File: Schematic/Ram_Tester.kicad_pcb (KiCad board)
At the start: 2 copper layers, 37.6 x 58.5 mm, 19 parts, among them J1 Conn_01x02_Pin, J2 ICSP, SW1 SW_DIP_x03, U1 ATmega328-P, U2 RAM, Y1 Crystal

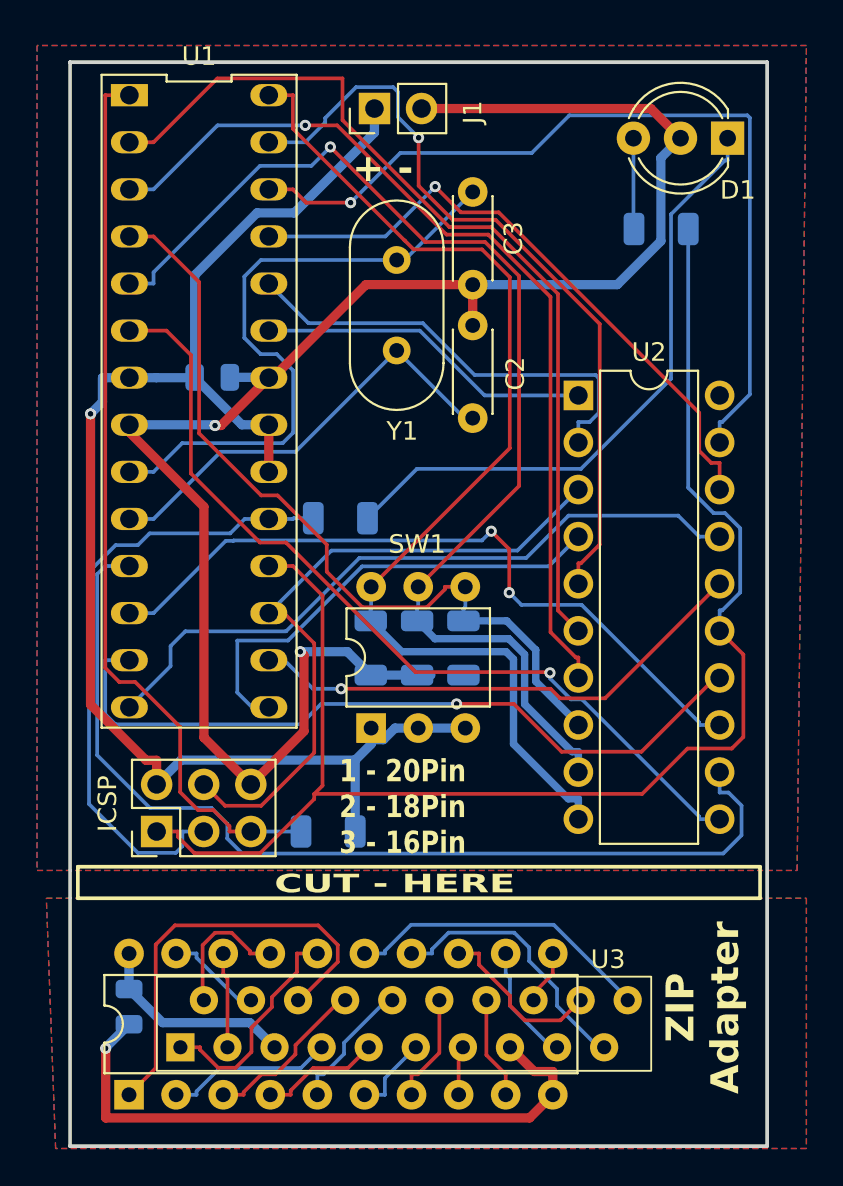
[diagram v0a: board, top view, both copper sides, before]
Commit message: v1.0 of PCB
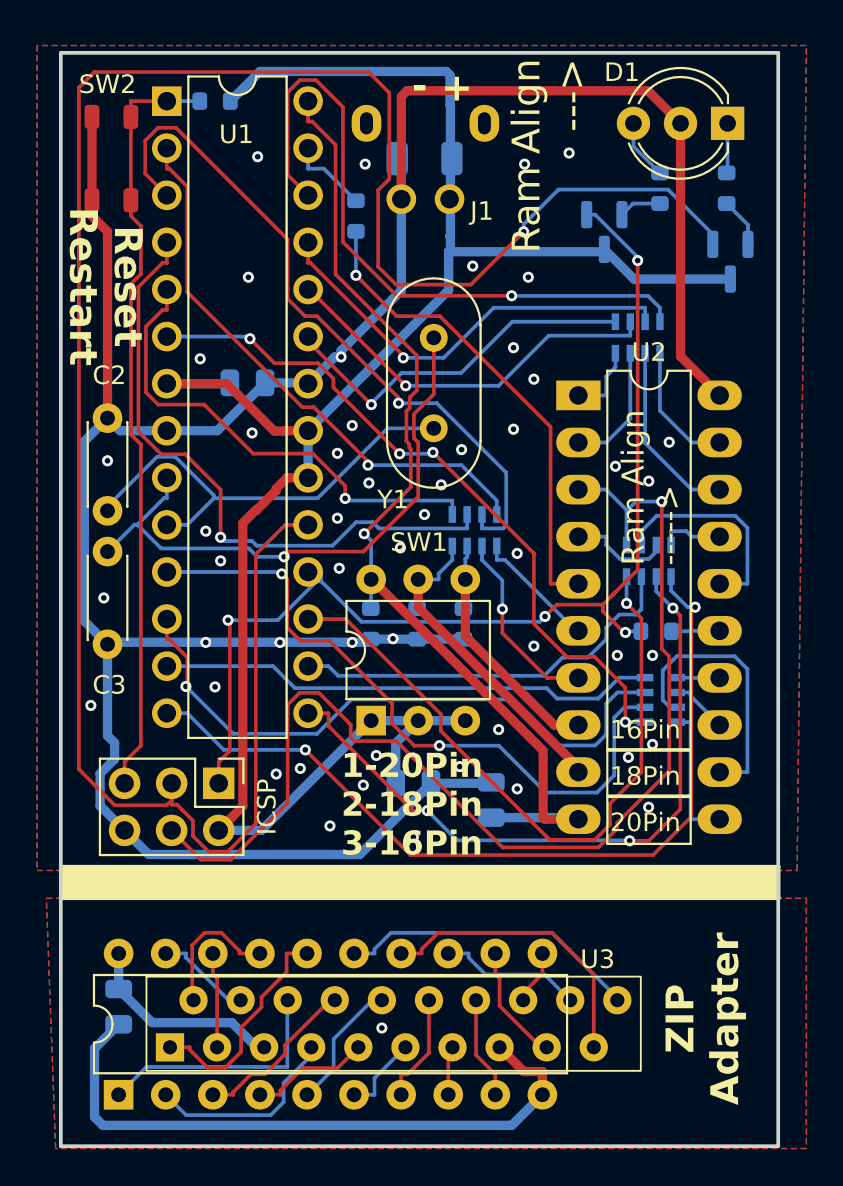
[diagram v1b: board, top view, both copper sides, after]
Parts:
- added C5: 10uF, Capacitor_SMD:C_1206_3216Metric, B.Cu at (124.9, 70.1)
- added C6: 100nF, Capacitor_SMD:C_0805_2012Metric, B.Cu at (128.5, 104.7)
- added C7: 100nF, Capacitor_SMD:C_0805_2012Metric, B.Cu at (124.3, 103.8)
- added Q1: IRLML6402, Package_TO_SOT_SMD:SOT-23, B.Cu at (134.6, 74.1)
- added Q2: IRLML6402, Package_TO_SOT_SMD:SOT-23, B.Cu at (141.4, 75.7)
- added R7: 47, Resistor_SMD:R_0603_1608Metric, B.Cu at (137.4, 95.6)
- added R8: 47, Resistor_SMD:R_0603_1608Metric, B.Cu at (121.2, 73.2)
- added RN1: 47, Resistor_SMD:R_Array_Concave_4x0603, B.Cu at (137.0, 91.8)
- added RN2: 47, Resistor_SMD:R_Array_Concave_4x0603, B.Cu at (137.7, 99.3)
- added RN3: 47, Resistor_SMD:R_Array_Concave_4x0603, B.Cu at (127.6, 90.2)
- added RN4: 47, Resistor_SMD:R_Array_Concave_4x0603, B.Cu at (136.4, 79.8)
- added SW2: SW_Push, Button_Switch_SMD:TLZWLA_Button, F.Cu at (100.3, 70.1)
- C2, C3: value 20pF -> 15pF
- J1: footprint Connector_PinHeader_2.54mm:PinHeader_1x02_P2.54mm_Vertical -> Connector_USB:MicroUSB PowerOnly
- R1, R2, R3, R4, R5, R6: footprint Resistor_SMD:R_1206_3216Metric -> Resistor_SMD:R_0603_1608Metric
- U1: footprint Package_DIP:ZIF-28 -> Package_DIP:DIP-28_W7.62mm
- U2: value RAM -> RAM / ZIF; footprint Package_DIP:ZIF-20 -> Package_DIP:DIP-20_W7.62mm_LongPads
- U3: value ~ -> ZIP Socket
- U4: value ~ -> DIP Socket
- moved R2 39.9 mm to (113.6, 67.0)
- moved C3 27.6 mm to (107.8, 91.3)
- moved R6 27.4 mm to (141.2, 71.7), turned to 90 degrees
- moved C2 20.3 mm to (107.8, 89.1)
- moved U1 16.3 mm to (111.0, 67.0), turned to 0 degrees
- moved J1 11.2 mm to (125.0, 78.3), turned to 180 degrees
- moved Y1 4.65 mm to (125.4, 84.7)
- moved J2 4.24 mm to (113.8, 103.8), turned to -90 degrees
- moved R1 2.20 mm to (137.6, 71.7), turned to -90 degrees
- moved C1 1.92 mm to (115.3, 82.2)
- moved R3 1.30 mm to (122.0, 95.2)
- moved R4 1.30 mm to (124.5, 95.2)
- moved R5 1.30 mm to (127.0, 95.2)
- moved D1 0.80 mm to (141.2, 68.2)
- moved U3 0.56 mm to (122.6, 110.4)
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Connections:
- R1 pad 1: Net-(J2-Pin_1) -> Net-(D1-K)
- R1 pad 2: Net-(D1-K) -> Net-(Q1-S)
- R4 pad 2: Net-(U1-PD3) -> Net-(RN3-R4.1)
- R5 pad 2: Net-(U1-PD2) -> Net-(RN3-R3.1)
- R6 pad 1: Net-(J2-Pin_3) -> Net-(Q2-S)
- SW1 pad 4: Net-(U1-PD2) -> Net-(RN3-R3.1)
- SW1 pad 5: Net-(U1-PD3) -> Net-(RN3-R4.1)
- U1 pad 11: Net-(U1-PD5) -> Net-(RN2-R3.2)
- U1 pad 12: Net-(U1-PD6) -> Net-(RN2-R2.2)
- U1 pad 13: Net-(U1-PD7) -> Net-(RN2-R1.2)
- U1 pad 14: Net-(U1-PB0) -> Net-(RN1-R4.2)
- U1 pad 15: Net-(U1-PB1) -> Net-(RN1-R3.2)
- U1 pad 16: Net-(U1-PB2) -> Net-(RN1-R2.2)
- U1 pad 17: Net-(J2-Pin_4) -> Net-(RN1-R1.2)
- U1 pad 2: Net-(U1-PD0) -> Net-(RN3-R1.2)
- U1 pad 23: Net-(U1-PC0) -> Net-(RN4-R4.2)
- U1 pad 24: Net-(U1-PC1) -> Net-(RN4-R3.2)
- U1 pad 25: Net-(U1-PC2) -> Net-(RN4-R2.2)
- U1 pad 26: Net-(U1-PC3) -> Net-(RN4-R1.2)
- U1 pad 3: Net-(U1-PD1) -> Net-(RN3-R2.2)
- U1 pad 4: Net-(U1-PD2) -> Net-(RN3-R3.2)
- U1 pad 5: Net-(U1-PD3) -> Net-(RN3-R4.2)
- U1 pad 6: Net-(U1-PD4) -> Net-(RN2-R4.2)
- U2 pad 1: Net-(U1-PC0) -> Net-(RN4-R4.1)
- U2 pad 11: Net-(U1-PD4) -> Net-(RN2-R4.1)
- U2 pad 12: Net-(U1-PD5) -> Net-(RN2-R3.1)
- U2 pad 13: Net-(U1-PD6) -> Net-(RN2-R2.1)
- U2 pad 14: Net-(U1-PD7) -> Net-(RN2-R1.1)
- U2 pad 15: Net-(J2-Pin_1) -> Net-(U2-A8)
- U2 pad 16: Net-(U1-PB2) -> Net-(RN1-R2.1)
- U2 pad 17: Net-(U1-PB0) -> Net-(RN1-R4.1)
- U2 pad 18: Net-(U1-PC2) -> Net-(RN4-R2.1)
- U2 pad 19: Net-(U1-PC3) -> Net-(RN4-R1.1)
- U2 pad 2: Net-(U1-PC1) -> Net-(RN4-R3.1)
- U2 pad 4: Net-(U1-PB1) -> Net-(RN1-R3.1)
- U2 pad 5: Net-(U1-PC4) -> Net-(U2-N/C)
- U2 pad 6: Net-(U1-PD0) -> Net-(RN3-R1.1)
- U2 pad 7: Net-(U1-PD1) -> Net-(RN3-R2.1)
- U2 pad 8: Net-(U1-PD2) -> Net-(RN3-R3.1)
- U2 pad 9: Net-(U1-PD3) -> Net-(RN3-R4.1)
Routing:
- net Net-(J2-Pin_3): track 34.0 -> 118.1 mm, vias 0 -> 1
- net Net-(U1-PD3): track 62.5 -> 0.00 mm, vias 1 -> 0
- net Net-(U1-PD5): track 53.7 -> 0.00 mm
- net /GND: track 96.0 -> 145.9 mm, vias 2 -> 51
- net Net-(U1-PD0): track 49.3 -> 0.00 mm
- net Net-(U1-PD1): track 49.2 -> 0.00 mm, vias 1 -> 0
- net Net-(U1-PD4): track 46.8 -> 0.00 mm, vias 1 -> 0
- net Net-(U1-PC3): track 46.5 -> 0.00 mm, vias 1 -> 0
- net Net-(RN1-R4.2): track 0.00 -> 46.1 mm, vias 0 -> 2
- net Net-(U1-PD2): track 44.0 -> 0.00 mm
- net Net-(U1-PD7): track 40.8 -> 0.00 mm, vias 1 -> 0
- net Net-(U1-PD6): track 39.5 -> 0.00 mm, vias 2 -> 0
- net Net-(RN2-R4.2): track 0.00 -> 38.1 mm, vias 0 -> 4
- net Net-(RN3-R2.2): track 0.00 -> 37.9 mm, vias 0 -> 1
- net Net-(U1-PB0): track 37.2 -> 0.00 mm
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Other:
- board size 37.6 x 58.5 mm -> 38.7 x 59 mm
- board text added: "1-20Pin 2-18Pin 3-16Pin"
- board text added: "16Pin"
- board text added: "18Pin"
- board text added: "20Pin"
- board text added: "Lower Side Towards ZIF"
- board text added: "Ram Align ----->"
- board text added: "Ram Align --->"
- board text added: "Reset Restart"
- board text added: "github.com/tops4u/Ram-Tester A.Hoffmann ©2024 License: GPL v3.0"
- board text removed: "1 - 20Pin 2 - 18Pin 3 - 16Pin"
- board text removed: "CUT - HERE"
- board text removed: "Lower Side Towards U2"
- board text removed: "RAM Tester (c) 2024 A.Hoffmann"
